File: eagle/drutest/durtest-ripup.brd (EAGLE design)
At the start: 100 x 80 mm, 70 parts, among them IC1 XCF02S, Q5 BC848SMD, Q6 BC848SMD, Q7 BC848SMD, Q8 BC848SMD, T1 BSS138, T2 BC848, T3 BSS138, U1 XC3S400TQ144, X1 1503_04, X2 SCART-F

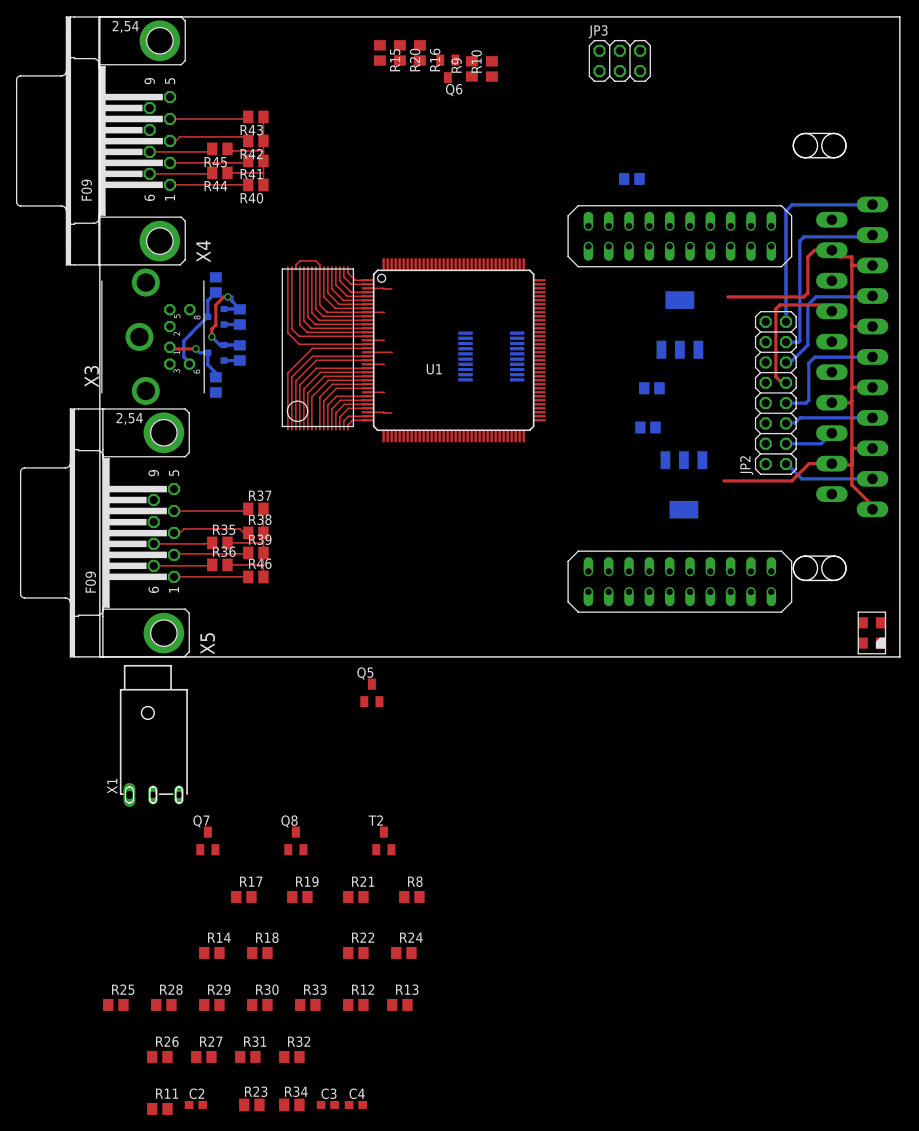
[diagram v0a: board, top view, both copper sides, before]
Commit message: hmmm
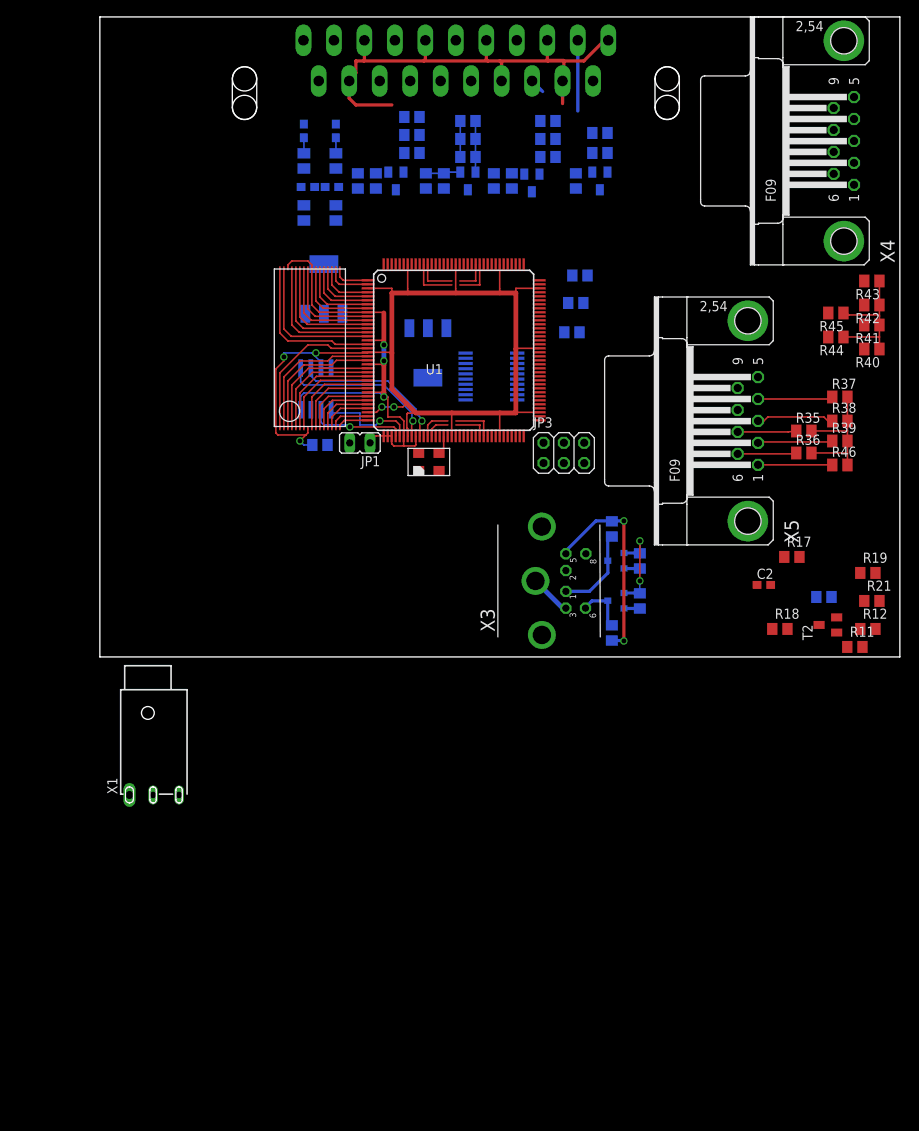
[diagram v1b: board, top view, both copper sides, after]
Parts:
- removed JP2: (no value), pinhead:2X08
- removed U$3: 2.5V, cpcfpga:SOT223
- removed U$4: 1.2V, cpcfpga:SOT223
- removed U$5: EXPHDR, cpcfpga:EXPHDR
- added C1, C5: (no value), resistor:C0603
- added IC2: 25LC080SN, microchip:SO-08
- added JP1: (no value), jumper:JP1
- added R47: 4K7, rcl:R0805
- added R48, R49: (no value), resistor:M0805
- added REG1.2: 1.2V, cpcfpga:SOT223
- added REG2.5: 2.5V, cpcfpga:SOT223
- moved R26 123.2 mm to (46.0, 67.0), flipped to the bottom, turned to 180 degrees
- moved C4 121.9 mm to (25.5, 65.8), flipped to the bottom, turned to 90 degrees
- moved C3 121.8 mm to (29.5, 65.8), flipped to the bottom, turned to 90 degrees
- moved R27 119.4 mm to (46.0, 64.8), flipped to the bottom, turned to 180 degrees
- moved R31 119.3 mm to (39.0, 67.5), flipped to the bottom
- moved R32 116.2 mm to (39.0, 65.2), flipped to the bottom
- moved R28 112.6 mm to (46.0, 62.5), flipped to the bottom, turned to 180 degrees
- moved R23 112.0 mm to (29.5, 55.5), flipped to the bottom, turned to 90 degrees
- moved R13 111.8 mm to (62.5, 65.5), flipped to the bottom, turned to 180 degrees
- moved R34 111.5 mm to (25.5, 55.5), flipped to the bottom, turned to 90 degrees
- moved R14 111.1 mm to (62.5, 63.0), flipped to the bottom, turned to 180 degrees
- moved R25 110.9 mm to (43.0, 59.5), flipped to the bottom, turned to 90 degrees
- moved R33 107.3 mm to (39.0, 63.0), flipped to the bottom
- moved R29 105.0 mm to (34.5, 59.5), flipped to the bottom, turned to 90 degrees
- moved R11 104.3 mm to (94.4, 1.25)
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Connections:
- removed net AOUTLEFT: JP2.13, R23.1, X2.3
- removed net AOUTRIGHT: JP2.15, R34.1, X2.1
- removed net AUDLEFT: C3.2
- removed net AUDRIGHT: C4.2
- removed net BLUE: JP2.11, X2.7
- removed net COMPOUT: JP2.1, X2.19
- removed net D_MODESWITCH: JP2.9, X2.8
- removed net GREEN: JP2.7, X2.11
- removed net N$66: U$2.OUT, U1.P55
- removed net RED: JP2.5, X2.15
- removed net VCC_B2: R22.1, R4.2, R6.2, T1.3, T2.3, T3.3
- new net FPGA_AUDIO_LEFT: R23.1
- new net FPGA_AUDIO_RIGHT: R34.1
- new net N$49: IC2.3, JP1.2, R47.1
- new net N$50: U$2.OUT, U1.P52
- new net N$51: C1.2, R23.2, R48.1
- new net N$52: C3.1, R48.2
- new net SPI_CLK: IC2.6, U1.P46
- new net SPI_DI: IC2.5, U1.P44
- new net SPI_DO: IC2.2, U1.P40
- new net SPI_SEL0: IC2.1, U1.P41
- net D_FASTBLANKING: no longer JP2.3, X2.16
- net GND: now also C1.1, C5.1, IC2.4, JP1.1, REG1.2.1, REG2.5.1; no longer U$3.1, U$4.1
- net N$64: now also C4.1, R49.2; no longer C3.1, R23.2
- net N$65: now also C5.2, R49.1; no longer C4.1
- net SCART_BLANKING: now also X2.16; no longer JP2.4
- net SCART_BLUE: now also X2.7; no longer JP2.12
- net SCART_COMP: now also X2.19; no longer JP2.2
- net SCART_GREEN: now also X2.11; no longer JP2.8
- net SCART_LEFT: now also C3.2, X2.3; no longer JP2.14
- net SCART_MODE: now also X2.8; no longer JP2.10
- net SCART_RED: now also X2.15; no longer JP2.6
- net SCART_RIGHT: now also C4.2, X2.1; no longer JP2.16
- net VCC: now also IC2.7, IC2.8, R22.1, R4.2, R47.2, R6.2, REG1.2.3, REG2.5.3, T1.3, T2.3, T3.3; no longer U$3.3, U$4.3
- net VCCAUX: now also REG2.5.4; no longer U$3.4
- net VCCINT: now also REG1.2.4; no longer U$4.4
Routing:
- net VCC: track 44.3 -> 181.5 mm, vias 0 -> 7
- net VCC_5V: track 0.00 -> 25.7 mm, vias 0 -> 2
- net AOUTRIGHT: track 25.0 -> 0.00 mm
- net GND: track 109.2 -> 133.5 mm, vias 0 -> 3
- net AOUTLEFT: track 23.7 -> 0.00 mm
- net VCCAUX: track 0.00 -> 20.6 mm
- net SPI_DI: track 0.00 -> 20.2 mm, vias 0 -> 1
- net SPI_CLK: track 0.00 -> 19.6 mm, vias 0 -> 1
- net D_MODESWITCH: track 17.6 -> 0.00 mm
- net BLUE: track 17.2 -> 0.00 mm
- net VCCINT: track 0.00 -> 16.5 mm
- net GREEN: track 15.9 -> 0.00 mm
- net VCC_B2: track 14.5 -> 0.00 mm, vias 2 -> 0
- net SPI_SEL0: track 0.00 -> 12.2 mm, vias 0 -> 1
- net SPI_DO: track 0.00 -> 12.2 mm, vias 0 -> 1
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
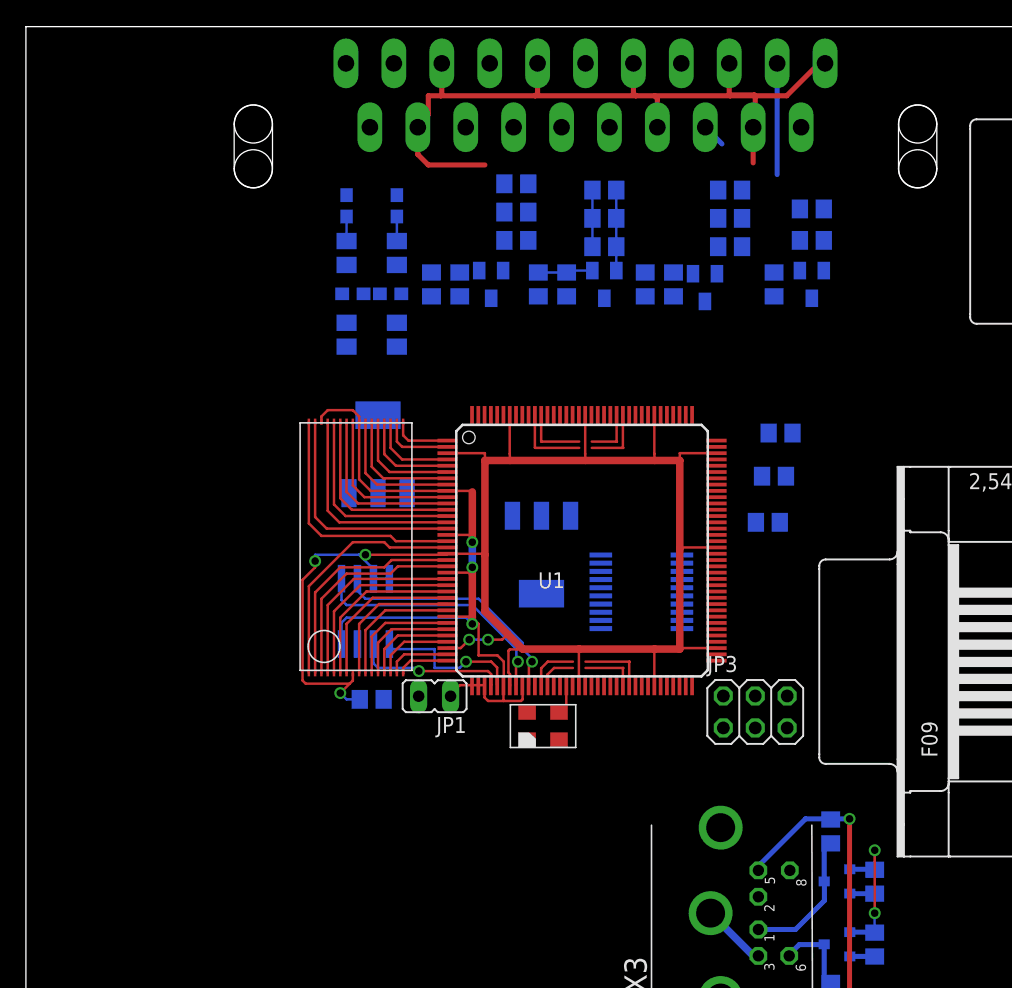
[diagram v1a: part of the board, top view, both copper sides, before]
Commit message: hmmm
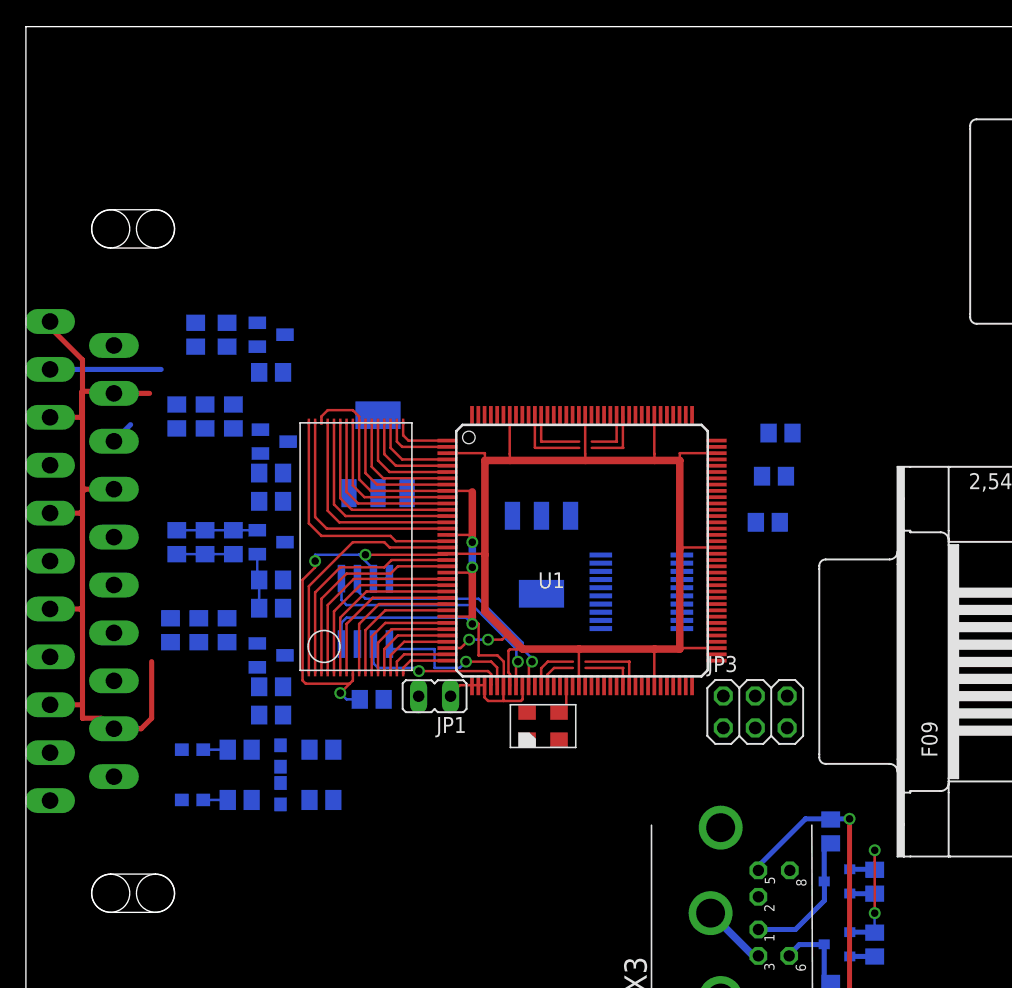
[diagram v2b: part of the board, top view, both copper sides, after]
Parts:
- moved X2 51.0 mm to (7.00, 37.5), turned to 270 degrees
- moved R13 50.0 mm to (13.5, 55.5), turned to 90 degrees
- moved C4 48.8 mm to (13.2, 18.5), turned to 0 degrees
- moved R15 47.5 mm to (12.0, 49.0), turned to 270 degrees
- moved R14 47.1 mm to (16.0, 55.5), turned to 90 degrees
- moved C3 46.2 mm to (13.2, 22.5), turned to 0 degrees
- moved R31 44.9 mm to (11.5, 32.0), turned to 270 degrees
- moved R20 44.6 mm to (14.2, 49.0), turned to 270 degrees
- moved R49 44.3 mm to (17.0, 18.5), turned to 0 degrees
- moved R26 44.0 mm to (12.0, 39.0), turned to 90 degrees
- moved Q5 43.2 mm to (19.5, 55.5), turned to 90 degrees
- moved R32 41.8 mm to (13.8, 32.0), turned to 270 degrees
- moved R16 41.7 mm to (16.5, 49.0), turned to 270 degrees
- moved R48 41.4 mm to (17.0, 22.5), turned to 0 degrees
- moved R27 40.9 mm to (14.2, 39.0), turned to 90 degrees
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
